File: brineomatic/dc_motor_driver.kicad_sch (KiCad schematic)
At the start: 6 parts, among them J18 3.5MM, J7 3.5MM, U4 DRV8871DDA

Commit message: updates parts, footprints, etc.  ready for production.
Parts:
- U4: LCSC C75864 -> (none); Mouser (none) -> 595-DRV8871DDAR
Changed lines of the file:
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@@
 			)
 		)
-		(property "LCSC" "C75864"
+		(property "LCSC" ""
 			(at 113.03 100.33 0)
 			(effects
+				(font
+					(size 1.27 1.27)
+				)
+				(hide yes)
+			)
+		)
+		(property "Mouser" " 595-DRV8871DDAR "
+			(at 113.03 100.33 0)
+			(effects

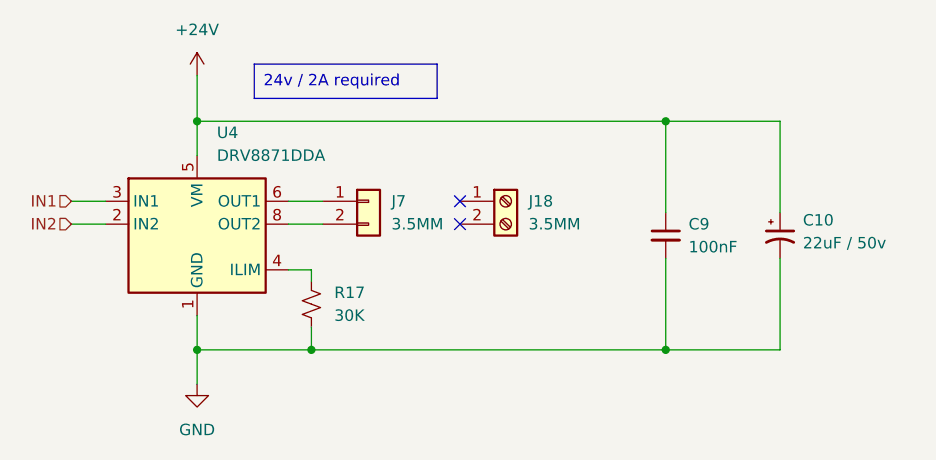
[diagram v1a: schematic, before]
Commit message: kicad v9 and updated todo.
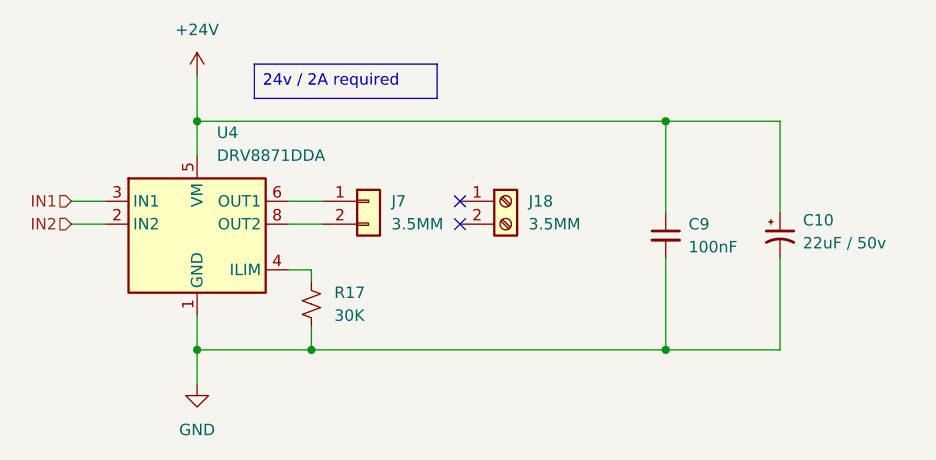
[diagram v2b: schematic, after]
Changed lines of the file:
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@@
 (kicad_sch
-	(version 20231120)
+	(version 20250114)
 	(generator "eeschema")
-	(generator_version "8.0")
+	(generator_version "9.0")
 	(paper "A4")
-	(junction
-		(at 125.73 114.3)
-		(diameter 0)
-		(color 0 0 0 0)
-	)
-	(junction
-		(at 113.03 88.9)
-		(diameter 0)
-		(color 0 0 0 0)
-	)
-	(junction
-		(at 165.1 114.3)
-		(diameter 0)
-		(color 0 0 0 0)
-	)
-	(junction
-		(at 113.03 114.3)
-		(diameter 0)
-		(color 0 0 0 0)
-	)
-	(junction
-		(at 165.1 88.9)
-		(diameter 0)
-		(color 0 0 0 0)
-	)
-	(no_connect
-		(at 142.24 100.33)
-	)
-	(no_connect
-		(at 142.24 97.79)
-	)
-	(wire
-		(pts
-			(xy 99.06 97.79) (xy 102.87 97.79)
-		)
-		(stroke
-			(width 0)
-			(type default)
-		)
-	)
-	(wire
-		(pts
-			(xy 125.73 114.3) (xy 165.1 114.3)
-		)
-		(stroke
-			(width 0)
-			(type default)
-		)
-	)
-	(wire
-		(pts
-			(xy 177.8 104.14) (xy 177.8 114.3)
-		)
-		(stroke
-			(width 0)
-			(type default)
-		)
-	)
-	(wire
-		(pts
-			(xy 177.8 88.9) (xy 177.8 99.06)
-		)
-		(stroke
-			(width 0)
-			(type default)
-		)
-	)
-	(wire
-		(pts
-			(xy 123.19 100.33) (xy 127 100.33)
-		)
-		(stroke
-			(width 0)
-			(type default)
-		)
-	)
-	(wire
-		(pts
-			(xy 177.8 114.3) (xy 165.1 114.3)
-		)
-		(stroke
-			(width 0)
-			(type default)
-		)
-	)
-	(wire
-		(pts
-			(xy 113.03 88.9) (xy 165.1 88.9)
-		)
-		(stroke
-			(width 0)
-			(type default)
-		)
-	)
-	(wire
-		(pts
-			(xy 123.19 105.41) (xy 125.73 105.41)
-		)
-		(stroke
-			(width 0)
-			(type default)
-		)
-	)
-	(wire
-		(pts
-			(xy 165.1 88.9) (xy 177.8 88.9)
-		)
-		(stroke
-			(width 0)
-			(type default)
-		)
-	)
-	(wire
-		(pts
-			(xy 123.19 97.79) (xy 127 97.79)
-		)
-		(stroke
-			(width 0)
-			(type default)
-		)
-	)
-	(wire
-		(pts
-			(xy 113.03 88.9) (xy 113.03 92.71)
-		)
-		(stroke
-			(width 0)
-			(type default)
-		)
-	)
-	(wire
-		(pts
-			(xy 99.06 100.33) (xy 102.87 100.33)
-		)
-		(stroke
-			(width 0)
-			(type default)
-		)
-	)
-	(wire
-		(pts
-			(xy 165.1 114.3) (xy 165.1 104.14)
-		)
-		(stroke
-			(width 0)
-			(type default)
-		)
-	)
-	(wire
-		(pts
-			(xy 113.03 110.49) (xy 113.03 114.3)
-		)
-		(stroke
-			(width 0)
-			(type default)
-		)
-	)
-	(wire
-		(pts
-			(xy 113.03 114.3) (xy 113.03 118.11)
-		)
-		(stroke
-			(width 0)
-			(type default)
-		)
-	)
-	(wire
-		(pts
-			(xy 113.03 114.3) (xy 125.73 114.3)
-		)
-		(stroke
-			(width 0)
-			(type default)
-		)
-	)
-	(wire
-		(pts
-			(xy 113.03 83.82) (xy 113.03 88.9)
-		)
-		(stroke
-			(width 0)
-			(type default)
-		)
-	)
-	(wire
-		(pts
-			(xy 125.73 111.76) (xy 125.73 114.3)
-		)
-		(stroke
-			(width 0)
-			(type default)
-		)
-	)
-	(wire
-		(pts
-			(xy 125.73 105.41) (xy 125.73 106.68)
-		)
-		(stroke
-			(width 0)
-			(type default)
-		)
-	)
-	(wire
-		(pts
-			(xy 165.1 88.9) (xy 165.1 99.06)
-		)
-		(stroke
-			(width 0)
-			(type default)
-		)
-	)
 	(text_box "24v / 2A required"
 		(exclude_from_sim no)
 		(at 119.38 82.55 0)
 		(size 20.32 3.81)
+		(margins 0.9525 0.9525 0.9525 0.9525)
 		(stroke
 			(width 0)
@@
 		)
 	)
+	(junction
+		(at 125.73 114.3)
+		(diameter 0)
+		(color 0 0 0 0)
+	)
+	(junction
+		(at 113.03 88.9)
+		(diameter 0)
+		(color 0 0 0 0)
+	)
+	(junction
+		(at 165.1 114.3)
+		(diameter 0)
+		(color 0 0 0 0)
+	)
+	(junction
+		(at 113.03 114.3)
+		(diameter 0)
+		(color 0 0 0 0)
+	)
+	(junction
+		(at 165.1 88.9)
+		(diameter 0)
+		(color 0 0 0 0)
+	)
+	(no_connect
+		(at 142.24 100.33)
+	)
+	(no_connect
+		(at 142.24 97.79)
+	)
+	(wire
+		(pts
+			(xy 99.06 97.79) (xy 102.87 97.79)
+		)
+		(stroke
+			(width 0)
+			(type default)
+		)
+	)
+	(wire
+		(pts
+			(xy 125.73 114.3) (xy 165.1 114.3)
+		)
+		(stroke
+			(width 0)
+			(type default)
+		)
+	)
+	(wire
+		(pts
+			(xy 177.8 104.14) (xy 177.8 114.3)
+		)
+		(stroke
+			(width 0)
+			(type default)
+		)
+	)
+	(wire
+		(pts
+			(xy 177.8 88.9) (xy 177.8 99.06)
+		)
+		(stroke
+			(width 0)
+			(type default)
+		)
+	)
+	(wire
+		(pts
+			(xy 123.19 100.33) (xy 127 100.33)
+		)
+		(stroke
+			(width 0)
+			(type default)
+		)
+	)
+	(wire
+		(pts
+			(xy 177.8 114.3) (xy 165.1 114.3)
+		)
+		(stroke
+			(width 0)
+			(type default)
+		)
+	)
+	(wire
+		(pts
+			(xy 113.03 88.9) (xy 165.1 88.9)
+		)
+		(stroke
+			(width 0)
+			(type default)
+		)
+	)
+	(wire
+		(pts
+			(xy 123.19 105.41) (xy 125.73 105.41)
+		)
+		(stroke
+			(width 0)
+			(type default)
+		)
+	)
+	(wire
+		(pts
+			(xy 165.1 88.9) (xy 177.8 88.9)
+		)
+		(stroke
+			(width 0)
+			(type default)
+		)
+	)
+	(wire
+		(pts
+			(xy 123.19 97.79) (xy 127 97.79)
+		)
+		(stroke
+			(width 0)
+			(type default)
+		)
+	)
+	(wire
+		(pts
+			(xy 113.03 88.9) (xy 113.03 92.71)
+		)
+		(stroke
+			(width 0)
+			(type default)
+		)
+	)
+	(wire
+		(pts
+			(xy 99.06 100.33) (xy 102.87 100.33)
+		)
+		(stroke
+			(width 0)
+			(type default)
+		)
+	)
+	(wire
+		(pts
+			(xy 165.1 114.3) (xy 165.1 104.14)
+		)
+		(stroke
+			(width 0)
+			(type default)
+		)
+	)
+	(wire
+		(pts
+			(xy 113.03 110.49) (xy 113.03 114.3)
+		)
+		(stroke
+			(width 0)
+			(type default)
+		)
+	)
+	(wire
+		(pts
+			(xy 113.03 114.3) (xy 113.03 118.11)
+		)
+		(stroke
+			(width 0)
+			(type default)
+		)
+	)
+	(wire
+		(pts
+			(xy 113.03 114.3) (xy 125.73 114.3)
+		)
+		(stroke
+			(width 0)
+			(type default)
+		)
+	)
+	(wire
+		(pts
+			(xy 113.03 83.82) (xy 113.03 88.9)
+		)
+		(stroke
+			(width 0)
+			(type default)
+		)
+	)
+	(wire
+		(pts
+			(xy 125.73 111.76) (xy 125.73 114.3)
+		)
+		(stroke
+			(width 0)
+			(type default)
+		)
+	)
+	(wire
+		(pts
+			(xy 125.73 105.41) (xy 125.73 106.68)
+		)
+		(stroke
+			(width 0)
+			(type default)
+		)
+	)
+	(wire
+		(pts
+			(xy 165.1 88.9) (xy 165.1 99.06)
+		)
+		(stroke
+			(width 0)
+			(type default)
+		)
+	)
 	(hierarchical_label "IN2"
 		(shape input)
 		(at 99.06 100.33 180)
-		(fields_autoplaced yes)
 		(effects
 			(font
@@
 		(shape input)
 		(at 99.06 97.79 180)
-		(fields_autoplaced yes)
 		(effects
 			(font
